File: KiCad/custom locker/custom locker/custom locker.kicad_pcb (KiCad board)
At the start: 2 copper layers, 8 parts, among them J1 servo motor connector, J3 HX711 load cell, SW1 SW_Push, SW2 SW_Push, SW3 SW_Push, U1 ESP32-DEVKITC-32D, U2 DM-OLED096-636

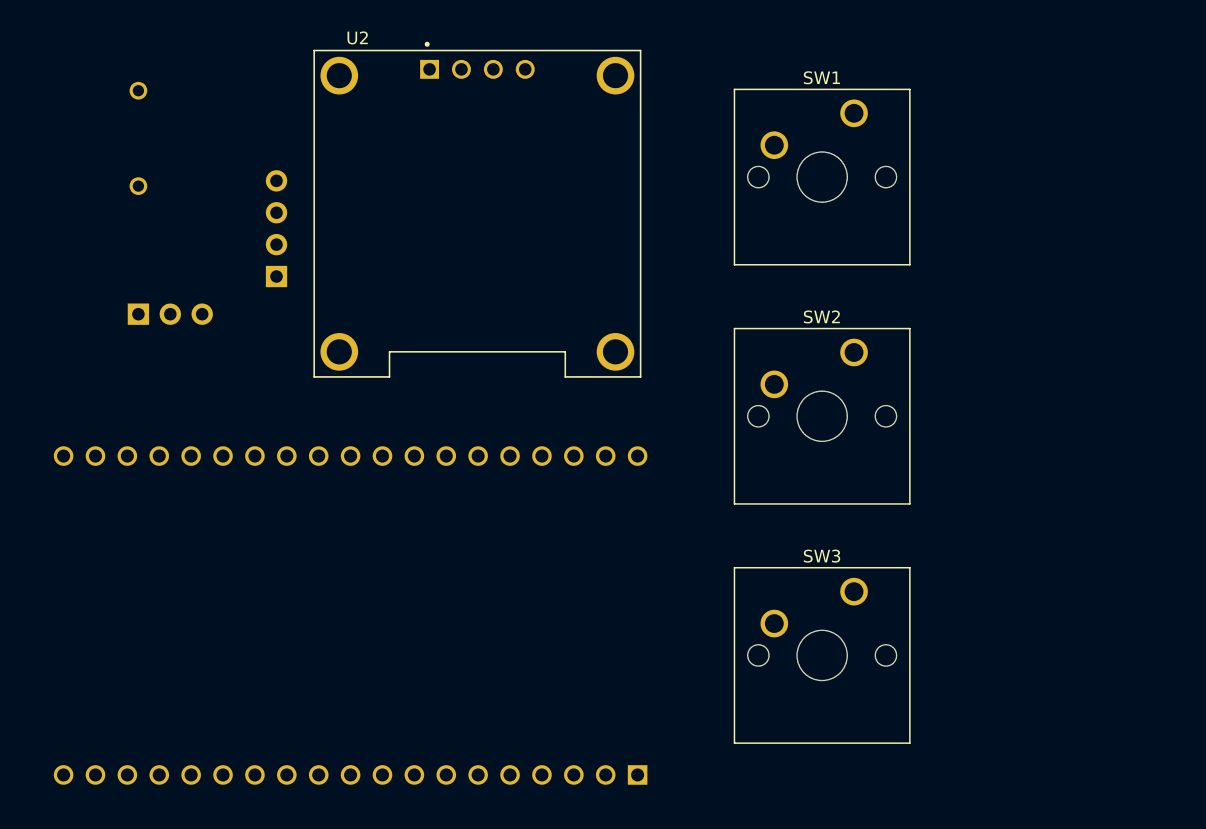
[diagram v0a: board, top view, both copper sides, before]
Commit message: finished pcb
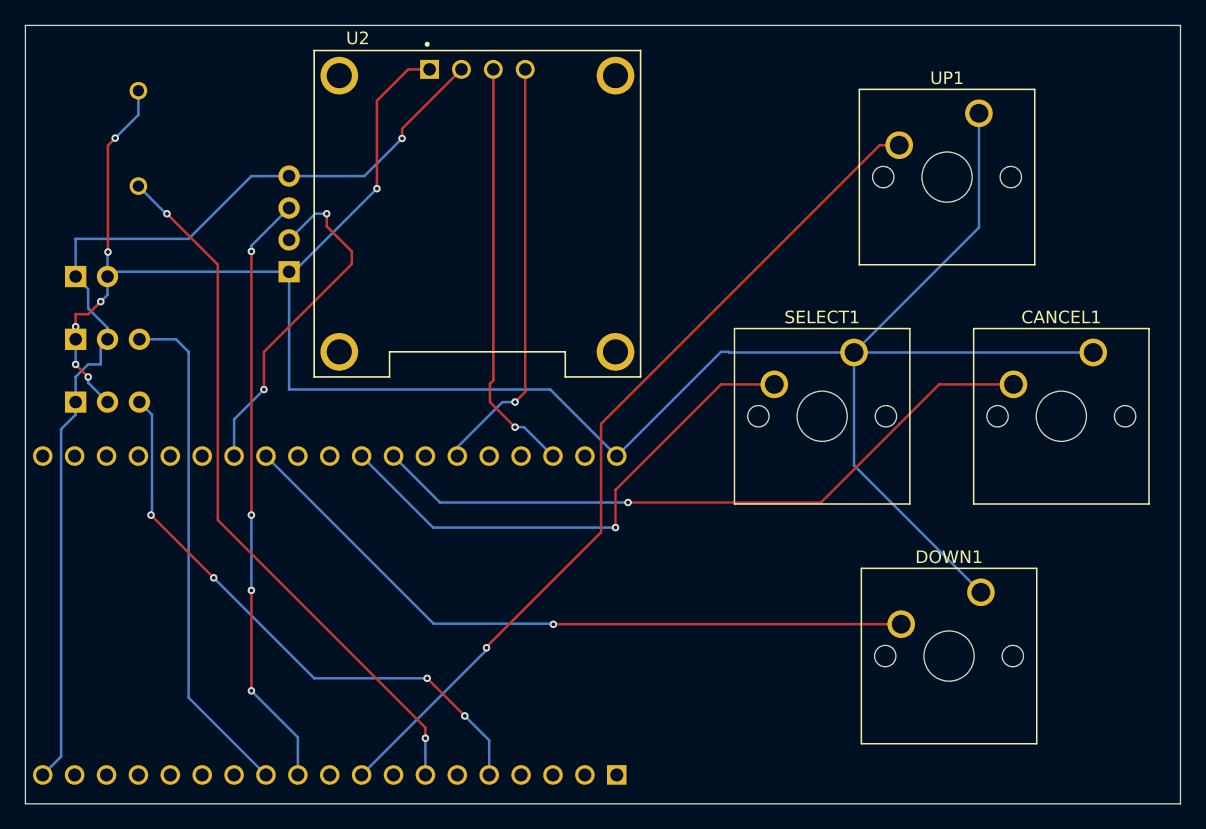
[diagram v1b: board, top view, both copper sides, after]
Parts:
- added DOWN1: SW_Push, Button_Switch_Keyboard:SW_Cherry_MX_1.00u_PCB, F.Cu at (88.1, 57.1)
- added J2: Power, Connector_PinHeader_2.54mm:PinHeader_1x02_P2.54mm_Vertical, B.Cu at (16.0, 32.0)
- added J4: Hall Effect Sensor, Connector_PinHeader_2.54mm:PinHeader_1x03_P2.54mm_Vertical, B.Cu at (16.0, 42.0)
- J1: value servo motor connector -> Servo Motor Connector
- moved CANCEL1 26.9 mm to (97.0, 38.0)
- moved UP1 9.95 mm to (87.9, 19.0)
- moved J1 5.39 mm to (16.0, 37.0)
- moved U1 1.66 mm to (39.3, 59.0)
- moved J3 1.07 mm to (33.0, 31.6)
- renumbered SW3 to CANCEL1, SW2 to SELECT1, SW1 to UP1
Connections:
- U1 pad J2-5: unconnected-(U1-IO34-PadJ2-5) -> Net-(J4-Pin_3)
- U1 pad J3-12: unconnected-(U1-IO16-PadJ3-12) -> SW4
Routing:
- net GND: track 0.00 -> 190.6 mm, vias 0 -> 7
- net +5V: track 0.00 -> 83.2 mm, vias 0 -> 1
- net SW1: track 0.00 -> 68.8 mm, vias 0 -> 1
- net Net-(U1-IO32): track 0.00 -> 56.4 mm, vias 0 -> 2
- net SW4: track 0.00 -> 56.2 mm, vias 0 -> 1
- net SW3: track 0.00 -> 54.8 mm, vias 0 -> 1
- net Clock: track 0.00 -> 47.9 mm, vias 0 -> 4
- net Net-(J4-Pin_3): track 0.00 -> 46.6 mm, vias 0 -> 4
- net SW2: track 0.00 -> 41.7 mm, vias 0 -> 1
- net Net-(J1-Pin_3): track 0.00 -> 40.6 mm
- net /I²C Data: track 0.00 -> 33.6 mm, vias 0 -> 1
- net /I²C Clock: track 0.00 -> 33.4 mm, vias 0 -> 1
- net /Data: track 0.00 -> 27.9 mm, vias 0 -> 2
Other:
- board outline added: 92 x 62 mm
